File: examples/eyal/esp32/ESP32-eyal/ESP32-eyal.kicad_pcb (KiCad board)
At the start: 2 copper layers, 47 x 45.7 mm, 31 parts, among them J1 Battery, J2 OW, J3 V1, J4 Serial, J5 VDD_I_SENSE, J6 BATT_I_SENSE, J7 ALT_V2, J8 ALT_V3, J9 Solar, Q1 2N7002W, Q2 DMP1045U, Q3 DMP1045U, Q4 DMP1045U, U1 RT9080-33, U2 ESP32-WROOM-32, U3 MCP73831

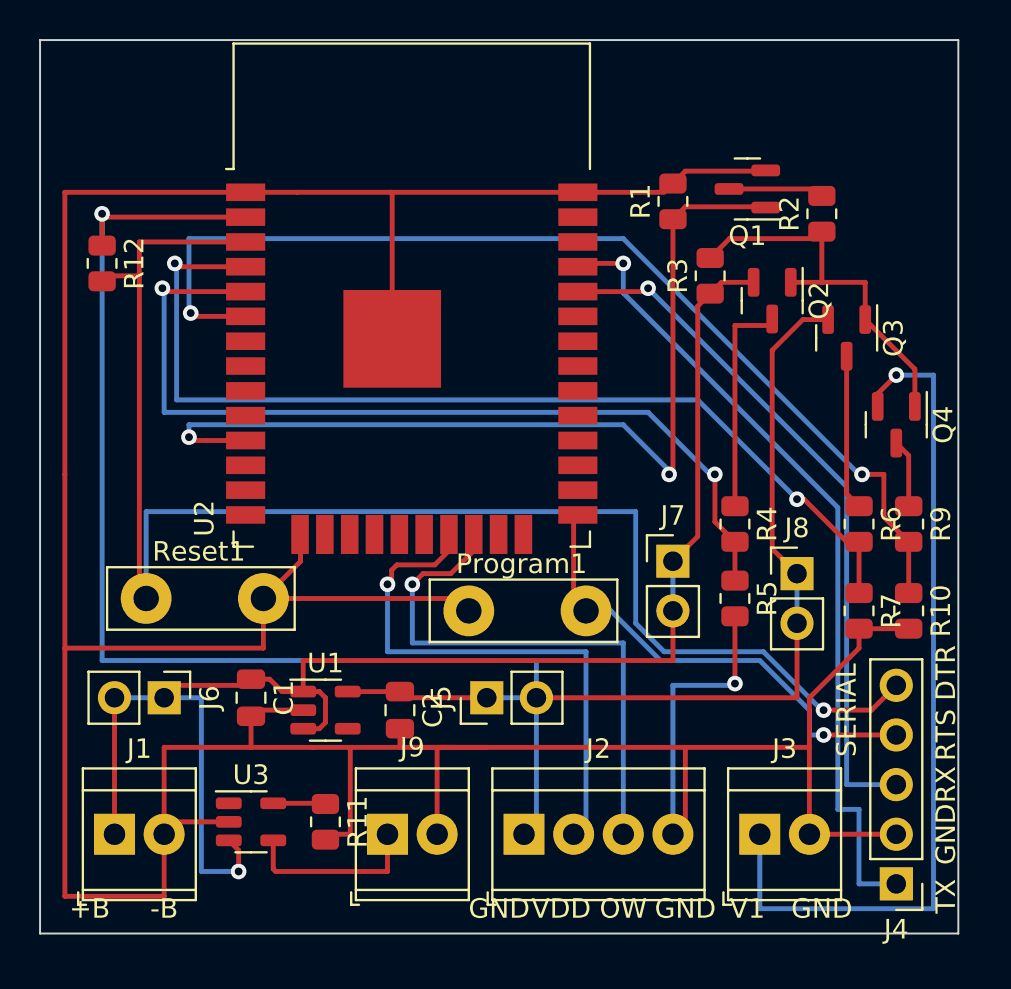
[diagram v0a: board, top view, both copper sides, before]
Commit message: some minor pcb adjustments (clear DRC warnings).
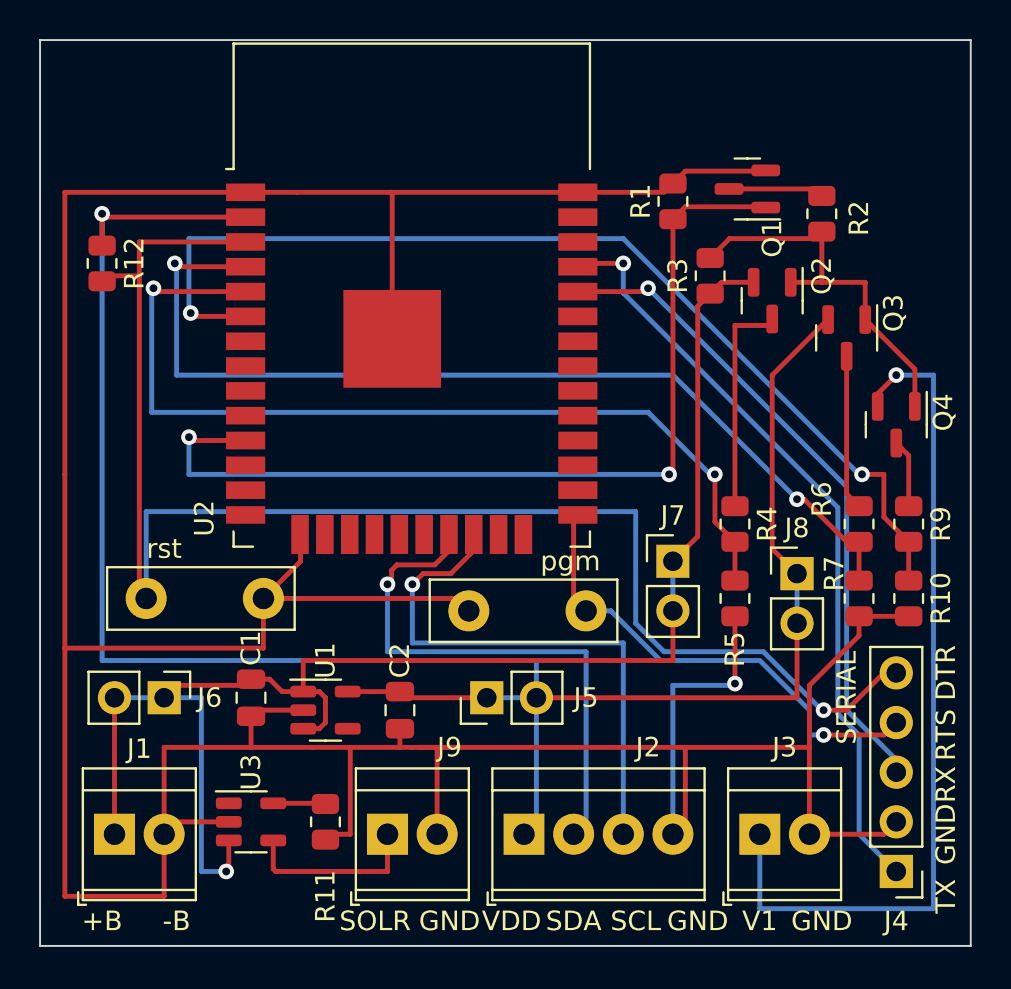
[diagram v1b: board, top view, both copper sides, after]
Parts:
- moved R10 0.64 mm to (139.7, 124.5)
- moved R7 0.64 mm to (137.2, 124.5)
- moved J4 0.63 mm to (139.1, 138.4)
- renumbered Program1 to pgm, Reset1 to rst
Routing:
- net Net-(J4-Pad1): track 41.4 -> 39.1 mm
- net Net-(J4-Pad3): track 35.6 -> 33.5 mm
- net GND: track 213.2 -> 211.6 mm
- net +BATT: track 78.5 -> 76.9 mm
- net /VDD_SENSE: track 51.3 -> 49.9 mm
- net VDD: track 108.7 -> 107.5 mm
- net /VBAT_SENSE: track 46.1 -> 47.2 mm
- net /V1_SENSE: track 53.9 -> 53.2 mm
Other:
- board size 47 x 45.7 mm -> 47.6 x 46.4 mm
- board text added: "SCL"
- board text added: "SDA"
- board text added: "SOLR"
- board text removed: "OW"
